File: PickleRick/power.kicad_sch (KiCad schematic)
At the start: 25 parts, among them J14 DeployLipo, J15 UCLipo, Q10 AO3401A, Q7 SI4143DY-T1-GE3, Q8 SI4143DY-T1-GE3, Q9 AO3401A, U10 LTC4411ES5TRMPBF, U11 LTC4411ES5TRMPBF, U12 LT1963AxST-3.3, U13 LTC4412xS6, U14 LTC4412xS6, U15 LTC4412xS6, U16 LTC4412xS6

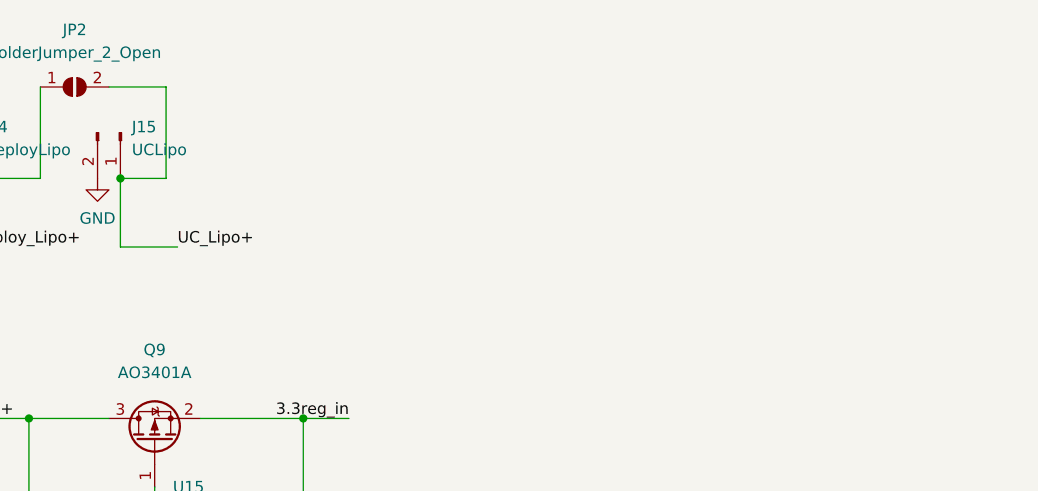
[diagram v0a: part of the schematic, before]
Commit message: pickle update
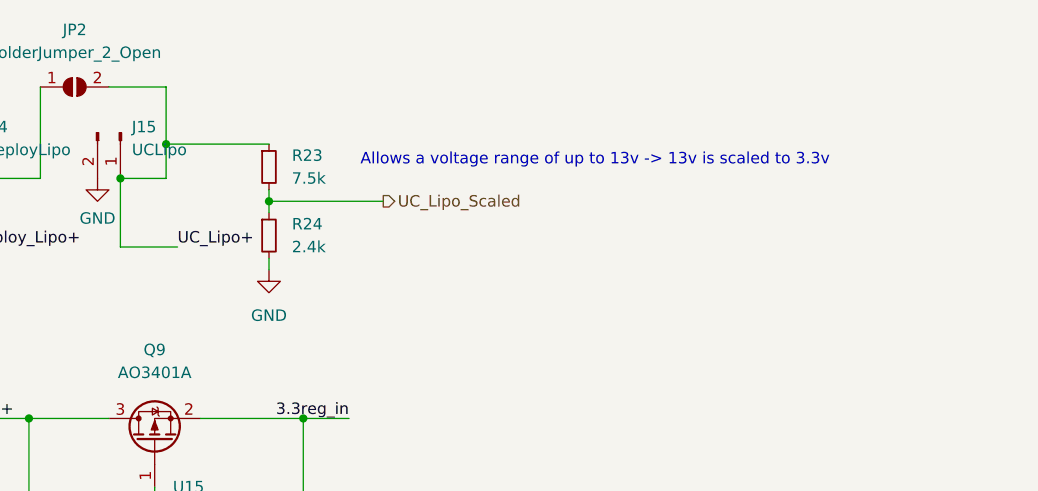
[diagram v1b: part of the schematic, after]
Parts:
- added R23: 7.5k, Resistor_SMD:R_0603_1608Metric, symbol Device:R_Small
- added R24: 2.4k, Resistor_SMD:R_0603_1608Metric, symbol Device:R_Small
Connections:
- net GND: now also R24.2
- net UC_Lipo+: now also R23.1
- new net UC_Lipo_Scaled: R23.2, R24.1
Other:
- note added: "Allows a voltage range of up to 13v -> 13v is scaled to 3.3v"
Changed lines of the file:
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@@
   (junction (at 205.74 39.37) (diameter 0) (color 0 0 0 0)
   )
+  (junction (at 222.25 41.91) (diameter 0) (color 0 0 0 0)
+  )
   (junction (at 195.58 66.04) (diameter 0) (color 0 0 0 0)
   )
@@
   )
   (junction (at 48.26 161.29) (diameter 0) (color 0 0 0 0)
+  )
+  (junction (at 210.82 35.56) (diameter 0) (color 0 0 0 0)
   )
   (no_connect (at 50.8 153.67))
@@
     (stroke (width 0) (type default) (color 0 0 0 0))
   )
+  (wire (pts (xy 222.25 48.26) (xy 222.25 49.53))
+    (stroke (width 0) (type default) (color 0 0 0 0))
+  )
   (wire (pts (xy 46.99 90.17) (xy 44.45 90.17))
     (stroke (width 0) (type default) (color 0 0 0 0))
@@
     (stroke (width 0) (type default) (color 0 0 0 0))
   )
+  (wire (pts (xy 210.82 35.56) (xy 210.82 39.37))
+    (stroke (width 0) (type default) (color 0 0 0 0))
+  )
   (wire (pts (xy 36.83 82.55) (xy 46.99 82.55))
     (stroke (width 0) (type default) (color 0 0 0 0))
@@
     (stroke (width 0) (type default) (color 0 0 0 0))
   )
-  (wire (pts (xy 210.82 29.21) (xy 210.82 39.37))
+  (wire (pts (xy 222.25 41.91) (xy 222.25 40.64))
+    (stroke (width 0) (type default) (color 0 0 0 0))
+  )
+  (wire (pts (xy 210.82 29.21) (xy 210.82 35.56))
     (stroke (width 0) (type default) (color 0 0 0 0))
   )
@@
     (stroke (width 0) (type default) (color 0 0 0 0))
   )
+  (wire (pts (xy 222.25 41.91) (xy 234.95 41.91))
+    (stroke (width 0) (type default) (color 0 0 0 0))
+  )
   (wire (pts (xy 48.26 156.21) (xy 48.26 161.29))
     (stroke (width 0) (type default) (color 0 0 0 0))
@@
     (stroke (width 0) (type default) (color 0 0 0 0))
   )
+  (wire (pts (xy 210.82 35.56) (xy 222.25 35.56))
+    (stroke (width 0) (type default) (color 0 0 0 0))
+  )
   (wire (pts (xy 50.8 148.59) (xy 55.88 148.59))
     (stroke (width 0) (type default) (color 0 0 0 0))
@@
     (stroke (width 0) (type default) (color 0 0 0 0))
   )
+  (wire (pts (xy 222.25 43.18) (xy 222.25 41.91))
+    (stroke (width 0) (type default) (color 0 0 0 0))
+  )
   (wire (pts (xy 119.38 142.24) (xy 129.54 142.24))
     (stroke (width 0) (type default) (color 0 0 0 0))
@@
   (wire (pts (xy 152.4 46.99) (xy 158.75 46.99))
     (stroke (width 0) (type default) (color 0 0 0 0))
+  )
+  (text "Allows a voltage range of up to 13v -> 13v is scaled to 3.3v"
+    (at 232.41 38.1 0)
+    (effects (font (size 1.27 1.27)) (justify left bottom))
   )
   (label "UC_Lipo+" (at 185.42 66.04 0)
@@
   (label "Deploy_Lipo+" (at 189.23 46.99 0)
     (effects (font (size 1.27 1.27)) (justify left bottom))
+  )
+  (hierarchical_label "UC_Lipo_Scaled" (shape output) (at 234.95 41.91 0)
+    (effects (font (size 1.27 1.27)) (justify left))
   )
   (hierarchical_label "RBUS_3.3_IN" (shape input) (at 33.02 148.59 180)
@@
     )
     (pin "1")
+  )
+  (symbol (lib_id "power:GND") (at 222.25 49.53 0) (unit 1)
+    (in_bom yes) (on_board yes) (fields_autoplaced)
+    (property "Reference" "#PWR039" (id 0) (at 222.25 55.88 0)
+      (effects (font (size 1.27 1.27)) hide)
+    )
+    (property "Value" "GND" (id 1) (at 222.25 54.61 0))
+    (property "Footprint" "" (id 2) (at 222.25 49.53 0)
+      (effects (font (size 1.27 1.27)) hide)
+    )
+    (property "Datasheet" "" (id 3) (at 222.25 49.53 0)
+      (effects (font (size 1.27 1.27)) hide)
+    )
+    (pin "1")
+  )
+  (symbol (lib_id "Device:R_Small") (at 222.25 38.1 0) (unit 1)
+    (in_bom yes) (on_board yes) (fields_autoplaced)
+    (property "Reference" "R23" (id 0) (at 224.79 36.8299 0)
+      (effects (font (size 1.27 1.27)) (justify left))
+    )
+    (property "Value" "7.5k" (id 1) (at 224.79 39.3699 0)
+      (effects (font (size 1.27 1.27)) (justify left))
+    )
+    (property "Footprint" "Resistor_SMD:R_0603_1608Metric" (id 2) (at 222.25 38.1 0)
+      (effects (font (size 1.27 1.27)) hide)
+    )
+    (property "Datasheet" "~" (id 3) (at 222.25 38.1 0)
+      (effects (font (size 1.27 1.27)) hide)
+    )
+    (pin "1")
+    (pin "2")
   )
   (symbol (lib_id "Mechanical:MountingHole_Pad") (at 41.91 43.18 0) (unit 1)
@@
     (pin "1")
   )
+  (symbol (lib_id "Device:R_Small") (at 222.25 45.72 0) (unit 1)
+    (in_bom yes) (on_board yes) (fields_autoplaced)
+    (property "Reference" "R24" (id 0) (at 224.79 44.4499 0)
+      (effects (font (size 1.27 1.27)) (justify left))
+    )
+    (property "Value" "2.4k" (id 1) (at 224.79 46.9899 0)
+      (effects (font (size 1.27 1.27)) (justify left))
+    )
+    (property "Footprint" "Resistor_SMD:R_0603_1608Metric" (id 2) (at 222.25 45.72 0)
+      (effects (font (size 1.27 1.27)) hide)
+    )
+    (property "Datasheet" "~" (id 3) (at 222.25 45.72 0)
+      (effects (font (size 1.27 1.27)) hide)
+    )
+    (pin "1")
+    (pin "2")
+  )
   (symbol (lib_id "power:GND") (at 41.91 99.06 0) (unit 1)
